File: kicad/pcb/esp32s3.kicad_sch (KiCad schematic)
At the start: 16 parts, among them J1 ESP JTAG, J3 ESP UART, SW1 ESP Boot, SW2 ESP Rst, U3 ESP32-S3-WROOM-2, Y2 32.768 KHz

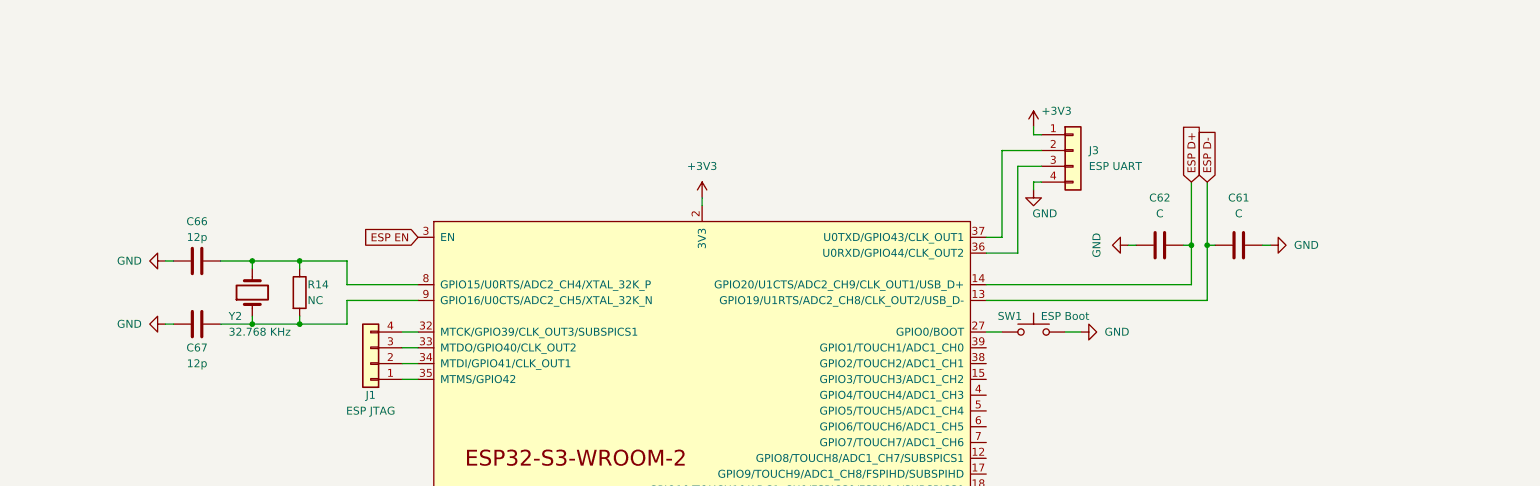
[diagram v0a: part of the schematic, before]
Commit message: (WIP) Tracing v2
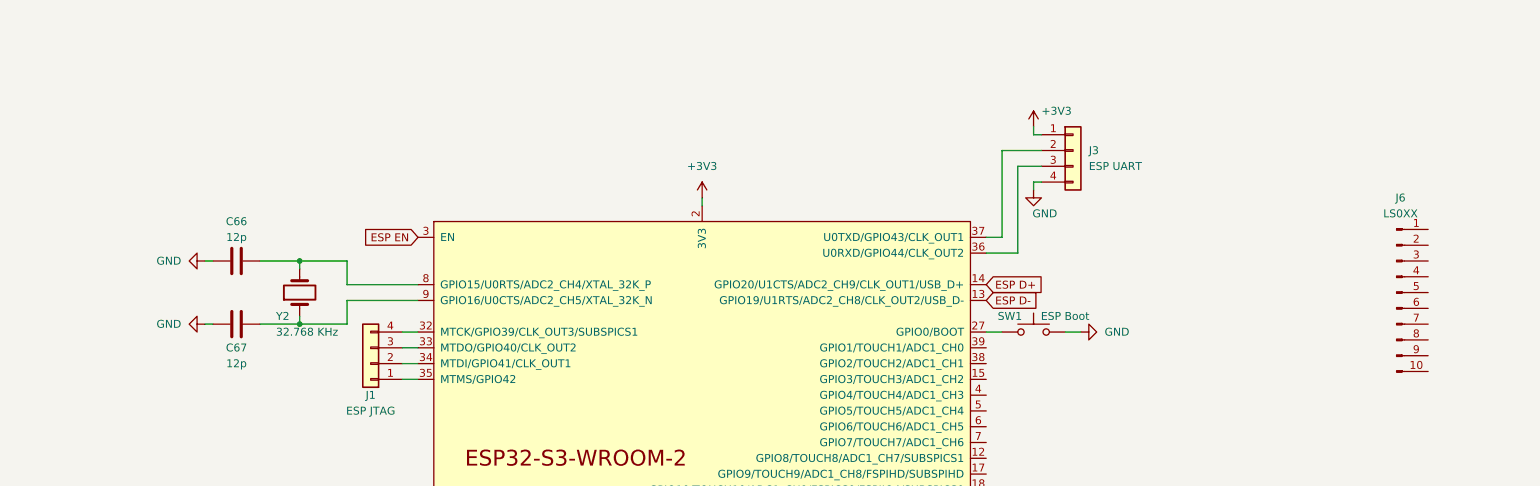
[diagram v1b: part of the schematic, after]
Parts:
- removed C61, C62: C, Capacitor_SMD:C_0402_1005Metric_Pad0.74x0.62mm_HandSolder, symbol Device:C
- removed R14: NC, Resistor_SMD:R_0402_1005Metric_Pad0.72x0.64mm_HandSolder, symbol Device:R
- added J6: LS0XX, Connector_FFC-FPC:Molex_54548-1071_1x10-1MP_P0.5mm_Horizontal, symbol Connector:Conn_01x10_Pin
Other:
- moved on the sheet: C66, C67, Y2
